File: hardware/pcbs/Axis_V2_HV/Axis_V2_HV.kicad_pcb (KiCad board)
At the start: 2 copper layers, 86.4 x 66 mm, 29 parts, among them J1 SWD, J2 UART, J3 Conn_01x02, J4 Conn_01x02, J5 Conn_01x04, J6 Conn_01x10, J7 Conn_01x08, SW1 RES, U1 Pico, U2 MAX31855EASA, U3 MAX31855EASA, U4 MAX6107, U5 FM24CL16B, U6 ADS1119IPWR, U7 TCA9534

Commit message: Updates to the HV pcb
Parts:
- removed C1, C2, C3, C4, C5: 0.1u, Capacitor_SMD:C_0402_1005Metric_Pad0.74x0.62mm_HandSolder
- removed J1: SWD, Connector_JST:JST_SH_BM03B-SRSS-TB_1x03-1MP_P1.00mm_Vertical
- removed J2: UART, Connector_JST:JST_SH_BM03B-SRSS-TB_1x03-1MP_P1.00mm_Vertical
- removed J3, J4: Conn_01x02, TerminalBlock_Phoenix:TerminalBlock_Phoenix_MKDS-1,5-2-5.08_1x02_P5.08mm_Horizontal
- removed J5: Conn_01x04, TerminalBlock_Phoenix:TerminalBlock_Phoenix_MKDS-1,5-4-5.08_1x04_P5.08mm_Horizontal
- removed J6: Conn_01x10, TerminalBlock_RND:TerminalBlock_RND_205-00240_1x10_P5.08mm_Horizontal
- removed J7: Conn_01x08, Connector_IDC:IDC-Header_2x04_P2.54mm_Vertical
- removed R1, R2, R3, R4, R5, R6, R7, R8, R9: 1k, Resistor_SMD:R_0402_1005Metric_Pad0.72x0.64mm_HandSolder
- removed SW1: RES, Button_Switch_SMD:SW_SPST_B3U-1000P
- removed U1: Pico, MCU_RaspberryPi_and_Boards:RPi_Pico_SMD_TH
- removed U2, U3: MAX31855EASA, Package_SO:SOIC-8_3.9x4.9mm_P1.27mm
- removed U4: MAX6107, Package_TO_SOT_SMD:SOT-23
- removed U5: FM24CL16B, Package_SO:SOIC-8_3.9x4.9mm_P1.27mm
- removed U6: ADS1119IPWR, Package_SO:TSSOP-16_4.4x5mm_P0.65mm
- removed U7: TCA9534, Package_SO:SOIC-16W_7.5x10.3mm_P1.27mm
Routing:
- net +3V3: track 178.4 -> 0.00 mm, vias 5 -> 0
- net /I2C0_SCL: track 78.0 -> 0.00 mm, vias 2 -> 0
- net /I2C0_SDA: track 73.5 -> 0.00 mm, vias 4 -> 0
- net /SPI0_RX: track 68.7 -> 0.00 mm, vias 4 -> 0
- net /SPI0_SCK: track 66.7 -> 0.00 mm, vias 4 -> 0
- net /SWDIO: track 52.6 -> 0.00 mm
- net /SPI0_CS1: track 48.6 -> 0.00 mm, vias 3 -> 0
- net /SWCLK: track 46.6 -> 0.00 mm
- net /SPI0_CS0: track 45.8 -> 0.00 mm, vias 4 -> 0
- net Net-(J7-Pin_7): track 44.4 -> 0.00 mm
- net +5V: track 41.2 -> 0.00 mm, vias 2 -> 0
- net Net-(J7-Pin_6): track 40.5 -> 0.00 mm
- net Net-(J7-Pin_5): track 37.5 -> 0.00 mm, vias 1 -> 0
- net /~{I2C0_ADS_RDY}: track 35.9 -> 0.00 mm, vias 4 -> 0
- net Net-(J7-Pin_4): track 33.5 -> 0.00 mm
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- removed copper zone on B.Cu, net GND
- removed copper zone on F.Cu, net GND
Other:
- board outline removed
- board text removed: "GP10"
- board text removed: "GP11"
- board text removed: "GP12"
- board text removed: "GP13"
- board text removed: "GP14"
- board text removed: "GP15"

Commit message: Is anyone listening anymore?
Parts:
- added C1: 10u, Capacitor_SMD:C_1206_3216Metric, B.Cu at (154.6, 56.6)
- added C2: 1n, Capacitor_SMD:C_1206_3216Metric, B.Cu at (152.0, 43.6)
- added C3: 0.1u, Capacitor_THT:C_Rect_L13.0mm_W6.0mm_P10.00mm_FKS3_FKP3_MKS4, F.Cu at (142.0, 46.0)
- added C4: 0.1u, Capacitor_THT:C_Rect_L13.0mm_W6.0mm_P10.00mm_FKS3_FKP3_MKS4, F.Cu at (116.0, 46.0)
- added C7: 0.1u, Capacitor_SMD:C_0402_1005Metric, B.Cu at (78.0, 79.0)
- added D1: MB6S, Package_TO_SOT_SMD:TO-269AA, B.Cu at (152.0, 49.0)
- added D2: 1N4148W, Diode_SMD:D_SOD-123, B.Cu at (149.8, 61.8)
- added F1: Fuse (3A, slow), Fuse:Fuseholder_Cylinder-5x20mm_Schurter_0031_8201_Horizontal_Open, F.Cu at (86.0, 40.0)
- added F2: Fuse (1A, Slow), Fuse:Fuseholder_Cylinder-5x20mm_Schurter_0031_8201_Horizontal_Open, F.Cu at (124.0, 62.5)
- added F3: Fuse (1A, Slow), Fuse:Fuseholder_Cylinder-5x20mm_Schurter_0031_8201_Horizontal_Open, F.Cu at (98.0, 62.5)
- added H1: MountingHole, MountingHole:MountingHole_2.7mm_M2.5, F.Cu at (64.0, 34.0)
- added H2: MountingHole, MountingHole:MountingHole_2.7mm_M2.5, F.Cu at (64.0, 86.0)
- added H3: MountingHole, MountingHole:MountingHole_2.7mm_M2.5, F.Cu at (156.0, 34.0)
- added H4: MountingHole, MountingHole:MountingHole_2.7mm_M2.5, F.Cu at (156.0, 86.0)
- added J1: Conn_01x08, Connector_IDC:IDC-Header_2x04_P2.54mm_Vertical, F.Cu at (86.2, 84.8)
- added J2: AC, TerminalBlock_Phoenix:TerminalBlock_Phoenix_MKDS-1,5-2-5.08_1x02_P5.08mm_Horizontal, F.Cu at (77.1, 36.0)
- added J3: PUMP, TerminalBlock_Phoenix:TerminalBlock_Phoenix_MKDS-1,5-2-5.08_1x02_P5.08mm_Horizontal, F.Cu at (139.5, 36.0)
- added J4: 3WAY, TerminalBlock_Phoenix:TerminalBlock_Phoenix_MKDS-1,5-2-5.08_1x02_P5.08mm_Horizontal, F.Cu at (113.0, 36.0)
- added J5: SSR, TerminalBlock_Phoenix:TerminalBlock_Phoenix_MKDS-1,5-2-5.08_1x02_P5.08mm_Horizontal, F.Cu at (65.7, 73.5)
- added J6: PWR, TerminalBlock_Phoenix:TerminalBlock_Phoenix_MKDS-1,5-2-5.08_1x02_P5.08mm_Horizontal, F.Cu at (65.8, 61.5)
- added OC1: 4N35, Package_DIP:SMDIP-6_W7.62mm, B.Cu at (152.0, 70.0)
- added Q1: MMBT3904, Package_TO_SOT_SMD:SOT-23, B.Cu at (153.4, 61.8)
- added Q2: BC847, Package_TO_SOT_SMD:SOT-23, B.Cu at (142.8, 80.5)
- added Q3: BC847, Package_TO_SOT_SMD:SOT-23, B.Cu at (126.0, 80.1)
- added R1: 1k, Resistor_SMD:R_0402_1005Metric, B.Cu at (109.0, 85.8)
- added R10: 220, Resistor_THT:R_Axial_DIN0207_L6.3mm_D2.5mm_P10.16mm_Horizontal, F.Cu at (142.0, 62.1)
- added R11: 1k, Resistor_SMD:R_0402_1005Metric, B.Cu at (141.8, 85.8)
- added R12: 162, Resistor_SMD:R_0603_1608Metric, B.Cu at (121.2, 79.6)
- added R13: 220, Resistor_THT:R_Axial_DIN0207_L6.3mm_D2.5mm_P10.16mm_Horizontal, F.Cu at (116.0, 62.1)
- added R14: 1k, Resistor_SMD:R_0402_1005Metric, B.Cu at (125.0, 83.6)
- added R2: 1k, Resistor_SMD:R_0402_1005Metric, B.Cu at (109.0, 83.2)
- added R3: 1k, Resistor_SMD:R_0402_1005Metric, B.Cu at (109.0, 81.2)
- added R4: 1k, Resistor_SMD:R_0402_1005Metric, B.Cu at (109.0, 79.2)
- added R5: 1k, LED_SMD:LED_1206_3216Metric, B.Cu at (150.6, 57.8)
- added R6: 220k, Resistor_THT:R_Axial_DIN0207_L6.3mm_D2.5mm_P10.16mm_Horizontal, F.Cu at (146.6, 48.8)
- added R7: 22k, Resistor_SMD:R_1206_3216Metric, B.Cu at (150.6, 55.0)
- added R8: 220k, Resistor_THT:R_Axial_DIN0207_L6.3mm_D2.5mm_P10.16mm_Horizontal, F.Cu at (157.4, 48.8)
- added R9: 162, Resistor_SMD:R_0603_1608Metric, B.Cu at (137.2, 79.0)
- added RV1: MOV-10D471K, Varistor:RV_Disc_D12mm_W7.5mm_P7.5mm, F.Cu at (137.0, 53.2)
- added RV2: MOV-10D471K, Varistor:RV_Disc_D12mm_W7.5mm_P7.5mm, F.Cu at (111.0, 53.2)
- added U1: AQH3213, Package_DIP:DIP-8-N7_W7.62mm, F.Cu at (134.2, 73.8)
- added U2: PCA9536DP, Package_SO:TSSOP-8_3x3mm_P0.65mm, B.Cu at (77.0, 83.8)
- added U3: AQH3213, Package_DIP:DIP-8-N7_W7.62mm, F.Cu at (108.2, 73.8)
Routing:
- net /AC_NEG: track 0.00 -> 69.5 mm
- net /AC_P: track 0.00 -> 64.0 mm
- net /PUMP_L: track 0.00 -> 36.2 mm
- net /3WAY_L: track 0.00 -> 36.0 mm
- net /AC_POS: track 0.00 -> 30.1 mm
- net Net-(F3-Pad1): track 0.00 -> 25.1 mm
- net Net-(F2-Pad1): track 0.00 -> 25.1 mm
- net Net-(D1--): track 0.00 -> 17.4 mm, vias 0 -> 2
- net Net-(OC1-Pad1): track 0.00 -> 9.82 mm
- net Net-(D1-+): track 0.00 -> 8.84 mm
- net Net-(C2-Pad2): track 0.00 -> 7.71 mm
- net Net-(C2-Pad1): track 0.00 -> 7.71 mm
- net Net-(D2-A): track 0.00 -> 7.13 mm
- net Net-(C4-Pad1): track 0.00 -> 5.92 mm
- net Net-(C3-Pad1): track 0.00 -> 5.92 mm
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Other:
- board outline added: 100 x 60 mm

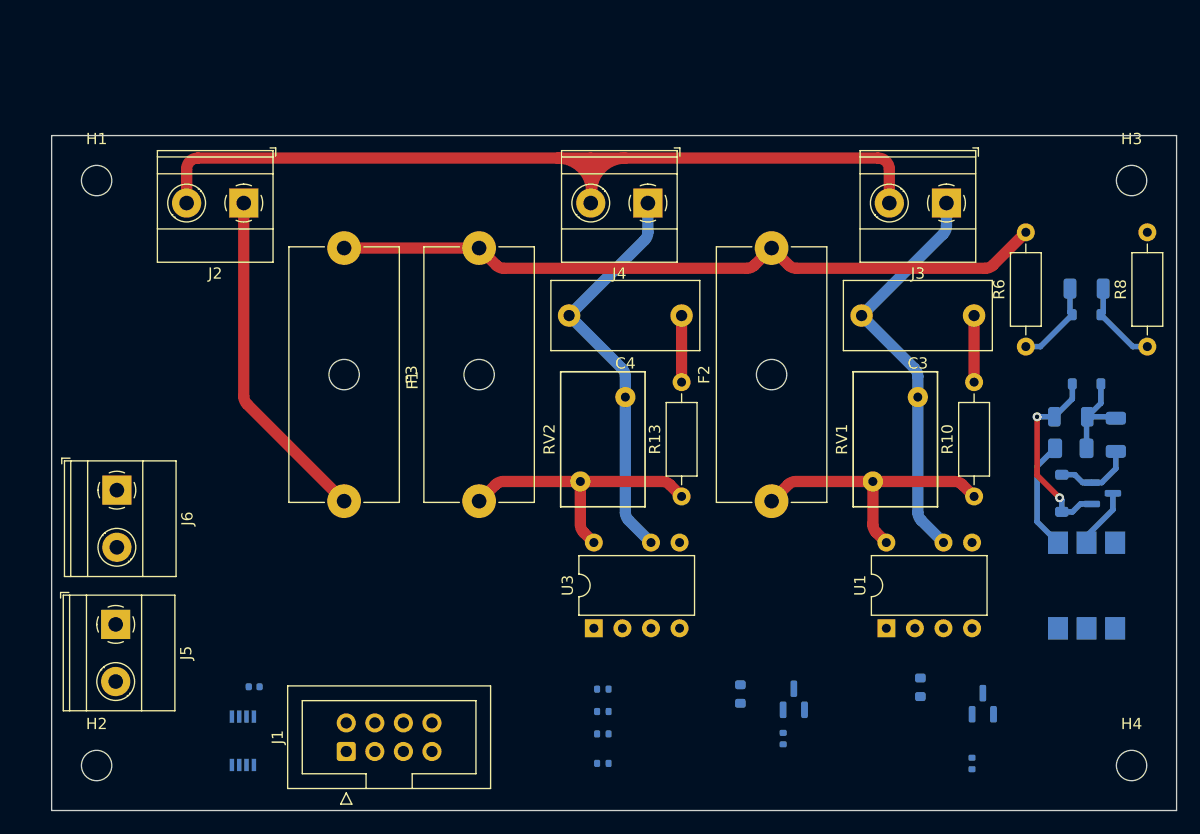
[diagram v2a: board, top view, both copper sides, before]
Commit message: Yuuuuuuuuuuuuuuuuuup, nobody's here
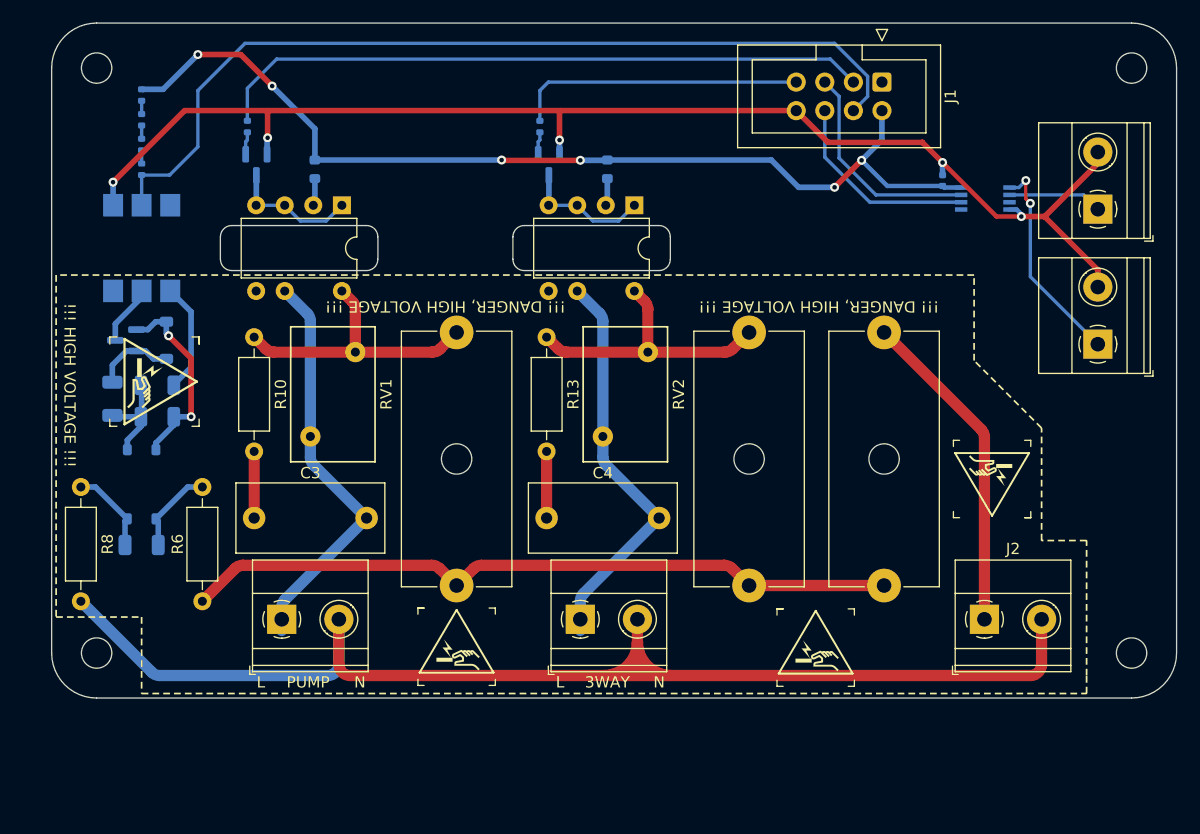
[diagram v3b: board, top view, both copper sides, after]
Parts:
- R5: footprint LED_SMD:LED_1206_3216Metric -> Resistor_SMD:R_1206_3216Metric
- moved H2 110.9 mm to (156.0, 24.0), turned to 180 degrees
- moved H4 110.9 mm to (64.0, 24.0), turned to 180 degrees
- moved H1 101.1 mm to (156.0, 76.0), turned to 180 degrees
- moved H3 101.1 mm to (64.0, 76.0), turned to 180 degrees
- moved R8 95.6 mm to (62.6, 61.2), turned to -90 degrees
- moved J5 94.8 mm to (153.0, 36.5), turned to 90 degrees
- moved C1 89.3 mm to (65.4, 53.4), turned to 90 degrees
- moved OC1 89.2 mm to (68.0, 40.0), turned to 90 degrees
- moved J6 88.2 mm to (153.0, 48.5), turned to 90 degrees
- moved Q1 87.9 mm to (66.6, 48.2), turned to 180 degrees
- moved C2 87.0 mm to (68.0, 66.4), turned to 180 degrees
- moved R11 85.8 mm to (77.4, 29.2), turned to -90 degrees
- moved D1 84.9 mm to (68.0, 61.0), turned to 90 degrees
- moved U2 81.7 mm to (143.0, 35.6), turned to 180 degrees
- moved R5 81.4 mm to (69.4, 52.2), turned to 0 degrees
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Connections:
- J1 pad 4: /ZC_SIG -> /~{ZC_SIG}
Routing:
- net GND: track 0.00 -> 117.6 mm, vias 0 -> 5
- net +3V3: track 0.00 -> 87.8 mm, vias 0 -> 6
- net /~{ZC_SIG}: track 0.00 -> 79.8 mm
- net /PUMP_IN: track 0.00 -> 58.7 mm
- net /AC_NEG: track 69.5 -> 103.6 mm
- net /3WAY_IN: track 0.00 -> 25.8 mm
- net /HV_SDA: track 0.00 -> 19.5 mm
- net /PWR_SW: track 0.00 -> 18.9 mm, vias 0 -> 2
- net /HV_SCL: track 0.00 -> 17.9 mm
- net Net-(Q3-C): track 0.00 -> 11.5 mm
- net Net-(Q2-C): track 0.00 -> 11.5 mm
- net /SSR: track 0.00 -> 8.38 mm
- net Net-(R9-Pad1): track 0.00 -> 2.43 mm
- net Net-(R12-Pad1): track 0.00 -> 2.43 mm
- net Net-(Q3-B): track 0.00 -> 2.01 mm
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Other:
- outline, holes or cut-outs redrawn
- board text added: "!!! DANGER, HIGH VOLTAGE !!!"
- board text added: "!!! HIGH VOLTAGE !!!"
- board text added: "3WAY"
- board text added: "L"
- board text added: "N"
- board text added: "PUMP"
